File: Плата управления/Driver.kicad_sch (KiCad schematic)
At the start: 25 parts

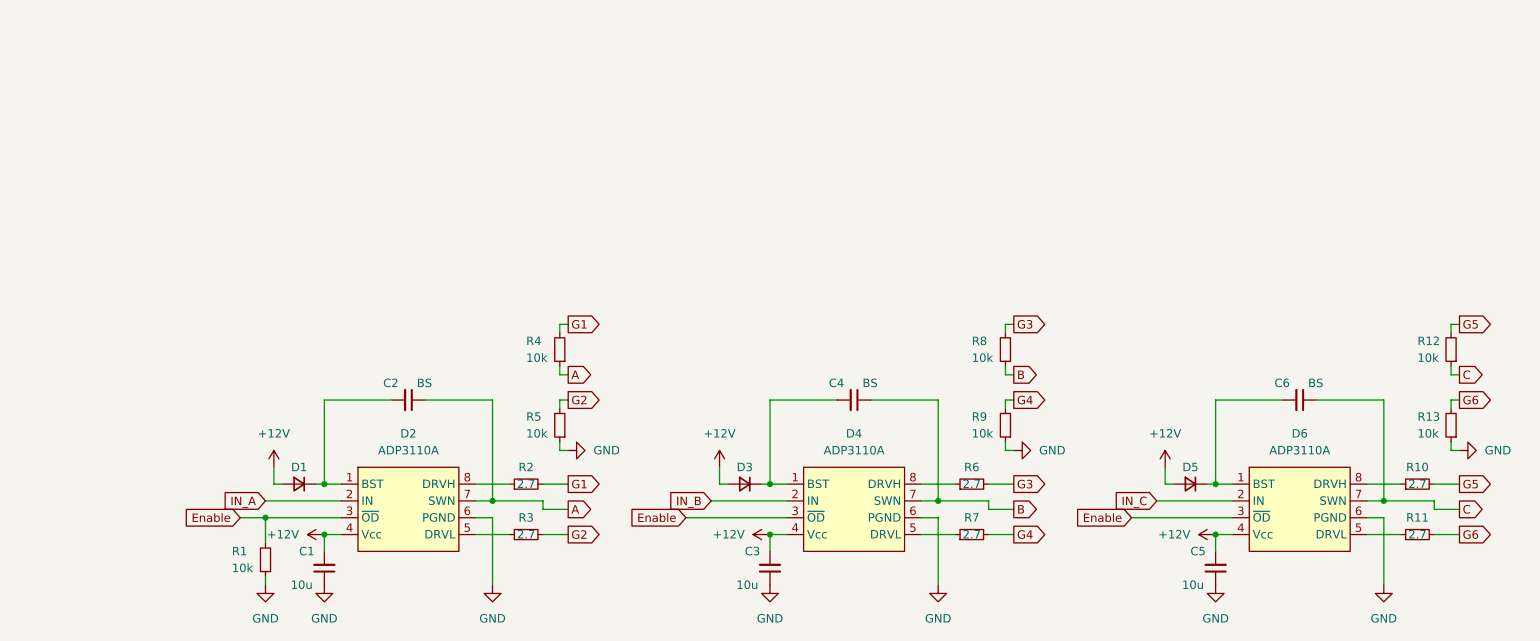
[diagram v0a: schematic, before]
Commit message: Привел в порядок схему
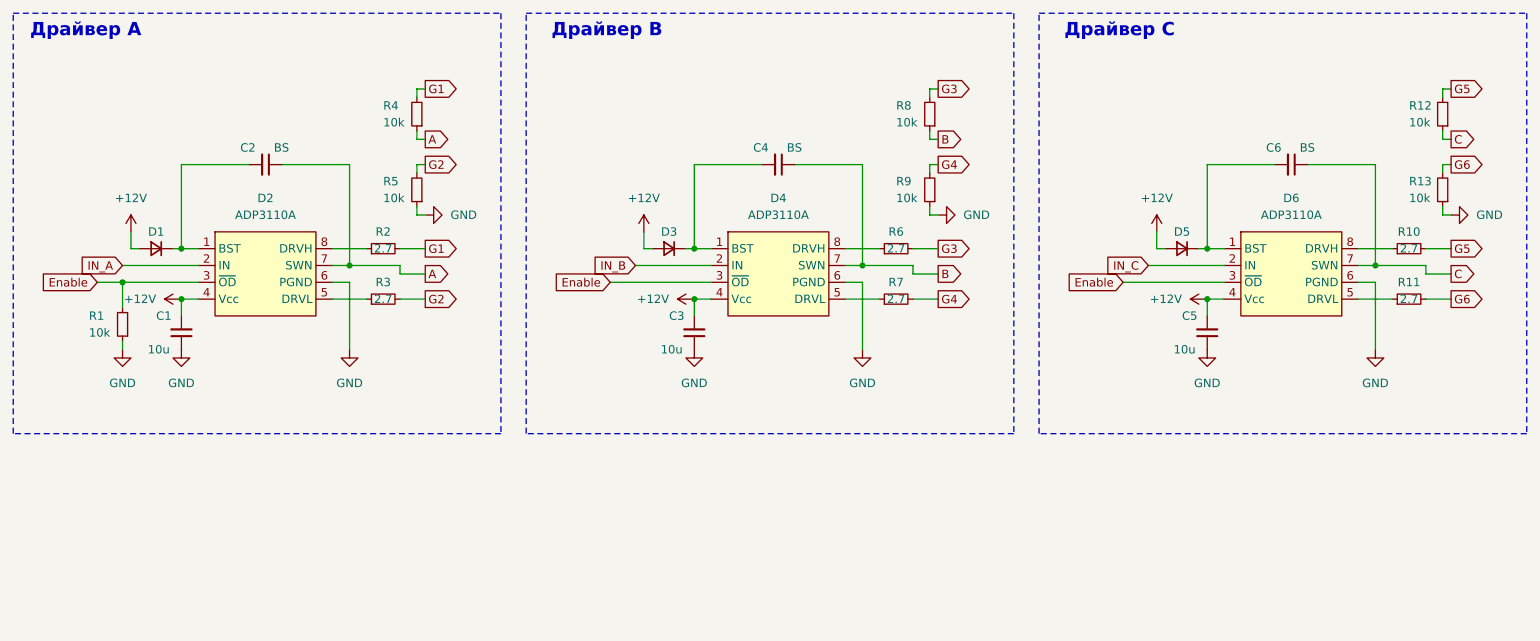
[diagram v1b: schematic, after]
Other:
- note added: "Драйвер А"
- note added: "Драйвер В"
- note added: "Драйвер С"
- moved on the sheet: C1, C2, C3, C4, C5, C6, D1, D2, D3, D4, D5, D6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

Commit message: Ещё нужно доработать
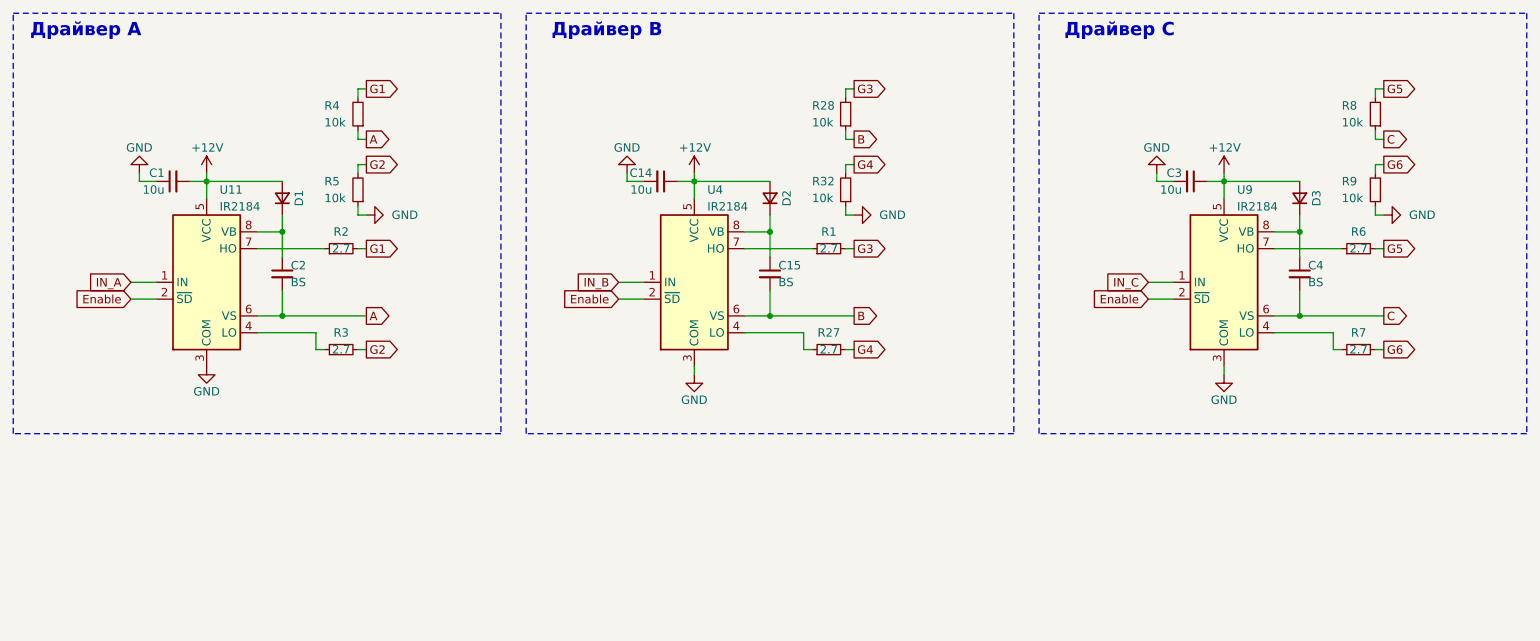
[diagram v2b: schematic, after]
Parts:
- removed C5: 10u, Capacitor_SMD:C_0603_1608Metric_Pad1.08x0.95mm_HandSolder, symbol Device:C_Small
- removed C6: BS, Capacitor_SMD:C_0805_2012Metric_Pad1.18x1.45mm_HandSolder, symbol Device:C_Small
- removed D2, D4, D6: ADP3110A, Package_DFN_QFN:DFN-8-1EP_3x3mm_P0.65mm_EP1.7x2.05mm, symbol IGBT_MOSFET_Drivers:ADP3110A
- removed D5: D_Small, Diode_SMD:D_SOD-323, symbol Device:D_Small
- removed R10, R11: 2.7, Resistor_SMD:R_0805_2012Metric_Pad1.20x1.40mm_HandSolder, symbol Device:R_Small
- removed R12, R13: 10k, Resistor_SMD:R_0603_1608Metric_Pad0.98x0.95mm_HandSolder, symbol Device:R_Small
- added C14: 10u, Capacitor_SMD:C_0603_1608Metric_Pad1.08x0.95mm_HandSolder, symbol Device:C_Small
- added C15: BS, Capacitor_SMD:C_0805_2012Metric_Pad1.18x1.45mm_HandSolder, symbol Device:C_Small
- added D2: D_Small, Diode_SMD:D_SOD-323, symbol Device:D_Small
- added R27: 2.7, Resistor_SMD:R_0805_2012Metric_Pad1.20x1.40mm_HandSolder, symbol Device:R_Small
- added R28, R32: 10k, Resistor_SMD:R_0603_1608Metric_Pad0.98x0.95mm_HandSolder, symbol Device:R_Small
- added U11, U4, U9: IR2184, Package_SO:SO-8_3.9x4.9mm_P1.27mm, symbol Driver_FET:IR2184
- R1: value 10k -> 2.7; footprint Resistor_SMD:R_0603_1608Metric_Pad0.98x0.95mm_HandSolder -> Resistor_SMD:R_0805_2012Metric_Pad1.20x1.40mm_HandSolder
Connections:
- net +12V: now also C3.1, C14.1, D2.2 (A), U11.5 (VCC), U4.5 (VCC), U9.5 (VCC); no longer C3.2
- net A: now also C2.2, U11.6 (VS); no longer C2.1
- net B: now also C15.2, R28.1, U4.6 (VS); no longer C4.1, R8.1
- net C: now also C4.2, R8.1, U9.6 (VS)
- net Enable: now also U11.2 (~{SD}), U4.2 (~{SD}), U9.2 (~{SD}); no longer R1.2
- net G3: now also R1.2, R28.2; no longer R6.2, R8.2
- net G4: now also R27.2, R32.2; no longer R7.2, R9.2
- net G5: now also R6.2, R8.2
- net G6: now also R7.2, R9.2
- net GND: now also C3.2, C14.2, R32.1, U11.3 (COM), U4.3 (COM), U9.3 (COM); no longer C3.1, R1.1
- net IN_A: now also U11.1 (IN)
- net IN_B: now also U4.1 (IN)
- net IN_C: now also U9.1 (IN)
- net at R2.1: now also U11.7 (HO)
- net at D1.1 (K): now also C2.1, U11.8 (VB); no longer C2.2
- net at R3.1: now also U11.4 (LO)
- net at D3.1 (K): now also C4.1, U9.8 (VB); no longer C4.2
- net at R6.1: now also U9.7 (HO)
- net at R7.1: now also U9.4 (LO)
- new net: R27.1, U4.4 (LO)
- new net: R1.1, U4.7 (HO)
- new net: C15.1, D2.1 (K), U4.8 (VB)
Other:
- moved on the sheet: C2, D1, R2, R3, R4, R5
